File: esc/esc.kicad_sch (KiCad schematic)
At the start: 45 parts, among them IC7 MA702GQ-P, U1 STM32G474RETx, Y1 NX2016SA-24M-EXS00A-CS08891

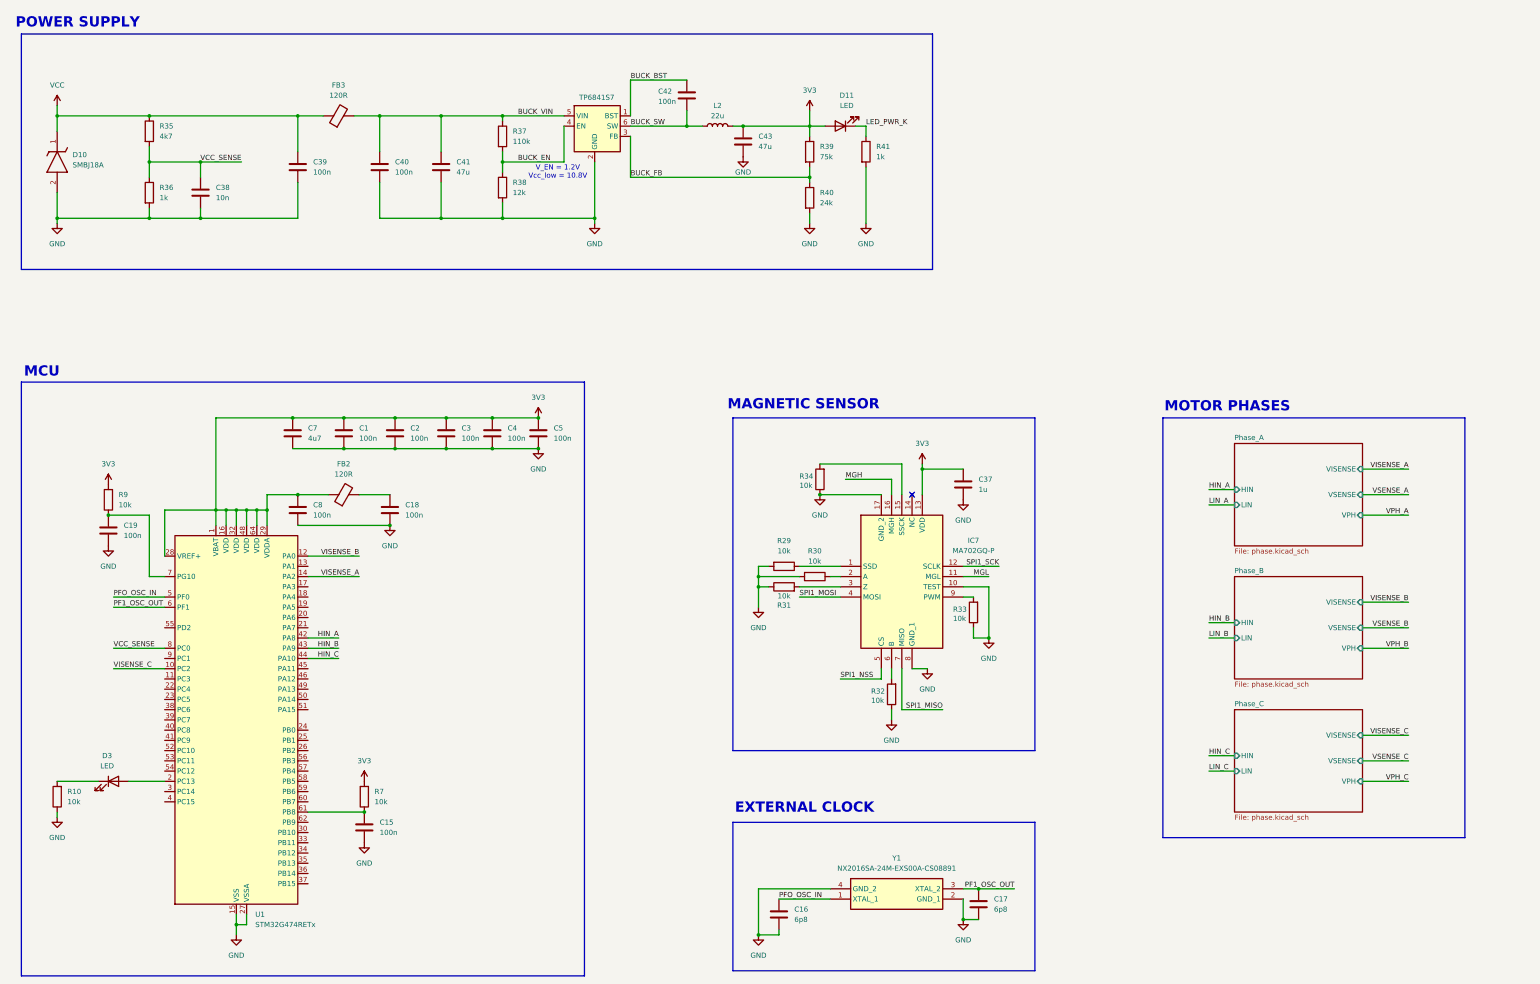
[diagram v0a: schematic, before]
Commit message: full layout
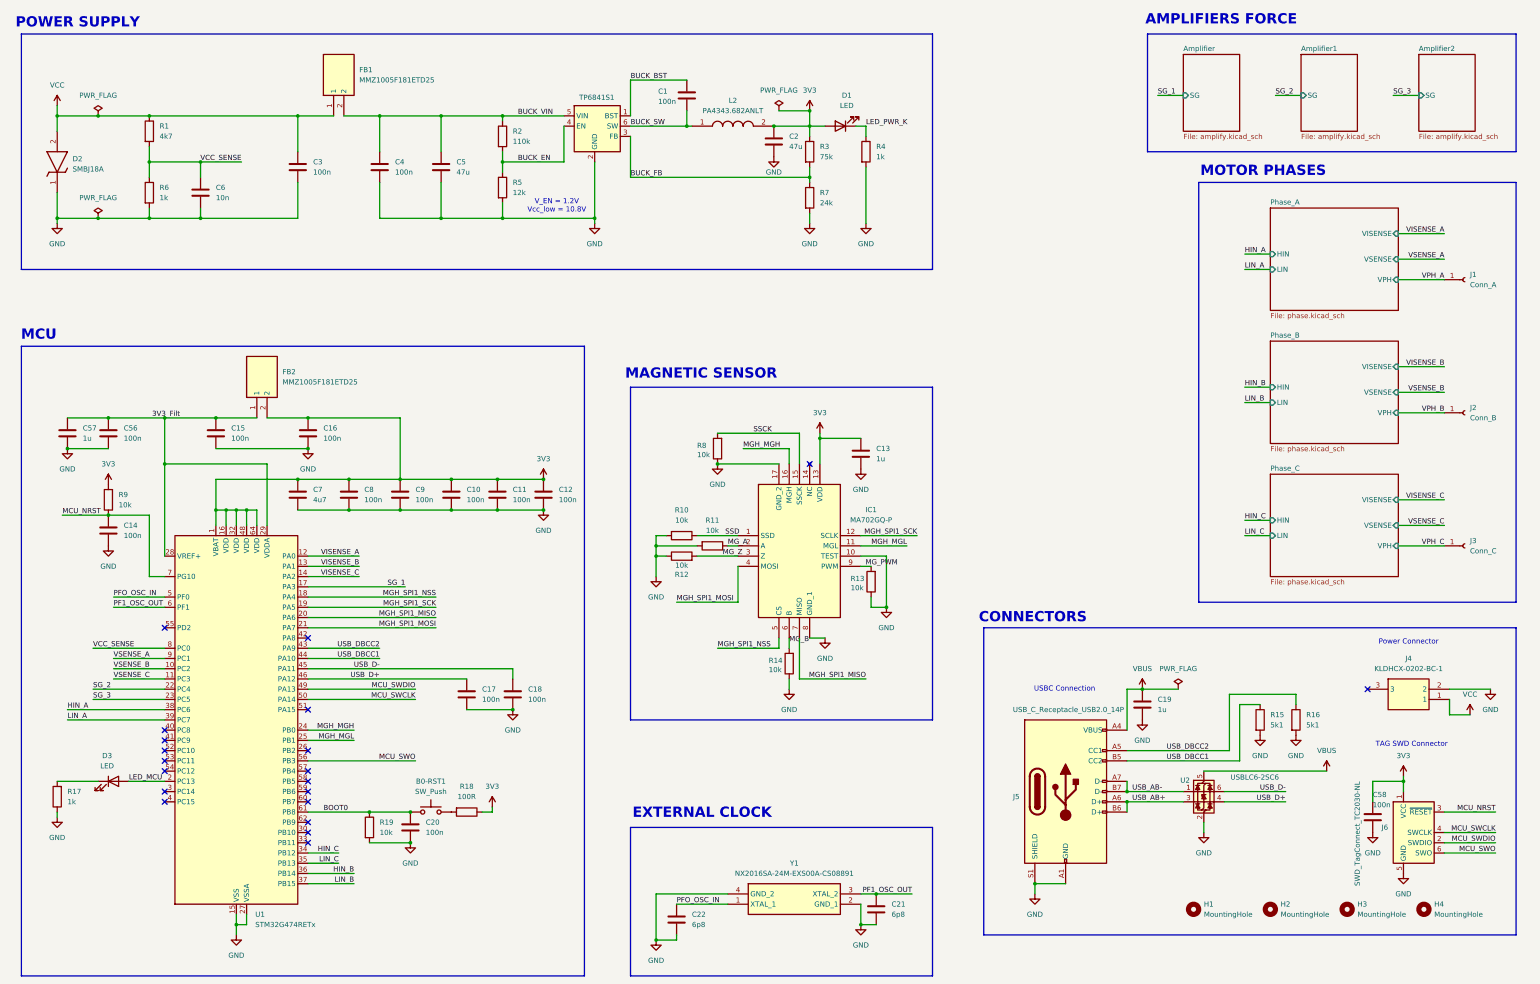
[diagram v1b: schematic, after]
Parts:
- removed D10: SMBJ18A, SamacSys_Parts:SMBJ18A, symbol SamacSys_Parts:SMBJ18A
- removed FB2, FB3: 120R, symbol Device:FerriteBead
- removed IC7: MA702GQ-P, QFN50P300X300X100-17N-D, symbol SamacSys_Parts:MA702GQ-P
- removed L2: 22u, symbol Device:L
- added B0-RST1: SW_Push, Button_Switch_SMD:SW_SPST_B3U-1000P, symbol Switch:SW_Push
- added C17, C18, C56, C58: 100n, Capacitor_SMD:C_0402_1005Metric, symbol Device:C
- added C19, C57: 1u, Capacitor_SMD:C_0603_1608Metric, symbol Device:C
- added D2: SMBJ18A, SamacSys_Parts:DIOM5436X244N, symbol SamacSys_Parts:SMBJ18A
- added FB1, FB2: MMZ1005F181ETD25, SamacSys_Parts:BEADC1005X55N, symbol SamacSys_Parts:MMZ1005F181ETD25
- added H1, H2, H3, H4: MountingHole, MountingHole:MountingHole_3.2mm_M3, symbol Mechanical:MountingHole
- added IC1: MA702GQ-P, SamacSys_Parts:QFN50P300X300X100-17N-D, symbol SamacSys_Parts:MA702GQ-P
- added J1: Conn_A, Connector_Wire:SolderWire-2sqmm_1x01_D2mm_OD3.9mm, symbol Connector:Conn_01x01_Socket
- added J2: Conn_B, Connector_Wire:SolderWire-2sqmm_1x01_D2mm_OD3.9mm, symbol Connector:Conn_01x01_Socket
- added J3: Conn_C, Connector_Wire:SolderWire-2sqmm_1x01_D2mm_OD3.9mm, symbol Connector:Conn_01x01_Socket
- added J4: KLDHCX-0202-BC-1, SamacSys_Parts:KLDHCX0202BC1, symbol SamacSys_Parts:KLDHCX-0202-BC-1
- added J5: USB_C_Receptacle_USB2.0_14P, Connector_USB:USB_C_Receptacle_Amphenol_12401610E4-2A, symbol Connector:USB_C_Receptacle_USB2.0_14P
- added J6: SWD_TagConnect_TC2030-NL, Connector:Tag-Connect_TC2030-IDC-NL_2x03_P1.27mm_Vertical, symbol Connector:Conn_ARM_SWD_TagConnect_TC2030-NL
- added L2: PA4343.682ANLT, SamacSys_Parts:INDPM135126X650N, symbol SamacSys_Parts:PA4343.682ANLT
- added R15, R16: 5k1, Resistor_SMD:R_0603_1608Metric, symbol Device:R
- added R19: 10k, Resistor_SMD:R_0603_1608Metric, symbol Device:R
- added U2: USBLC6-2SC6, Package_TO_SOT_SMD:SOT-23-6, symbol Power_Protection:USBLC6-2SC6
- C1: renamed from C42; footprint (none) -> Capacitor_SMD:C_0402_1005Metric; Link (none) -> https://www.mouser.de/ProductDetail/Murata-Electronics/GRM0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; MF (none) -> Murata Electronics; MP (none) -> GRM02YR60G104ME01L; MPN (none) -> 81-GRM02YR60G104ME1L
- C10: renamed from C3; footprint (none) -> Capacitor_SMD:C_0402_1005Metric; Link (none) -> https://www.mouser.de/ProductDetail/Murata-Electronics/GRM0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; MF (none) -> Murata Electronics; MP (none) -> GRM02YR60G104ME01L; MPN (none) -> 81-GRM02YR60G104ME1L
- C11: renamed from C4; footprint (none) -> Capacitor_SMD:C_0402_1005Metric; Link (none) -> https://www.mouser.de/ProductDetail/Murata-Electronics/GRM0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; MF (none) -> Murata Electronics; MP (none) -> GRM02YR60G104ME01L; MPN (none) -> 81-GRM02YR60G104ME1L
- C12: renamed from C5; footprint (none) -> Capacitor_SMD:C_0402_1005Metric; Link (none) -> https://www.mouser.de/ProductDetail/Murata-Electronics/GRM0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; MF (none) -> Murata Electronics; MP (none) -> GRM02YR60G104ME01L; MPN (none) -> 81-GRM02YR60G104ME1L
- C13: renamed from C37; footprint (none) -> Capacitor_SMD:C_0603_1608Metric; Link (none) -> https://www.mouser.de/ProductDetail/TAIYO-YUDEN/MBJCT168CB7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; MF (none) -> TAIYO YUDEN; MP (none) -> MBJCT168CB7105KRPA01; MPN (none) -> 963-BJCT168CB7105KR
- C14: renamed from C19; footprint (none) -> Capacitor_SMD:C_0402_1005Metric; Link (none) -> https://www.mouser.de/ProductDetail/Murata-Electronics/GRM0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; MF (none) -> Murata Electronics; MP (none) -> GRM02YR60G104ME01L; MPN (none) -> 81-GRM02YR60G104ME1L
- C15: renamed from C8; footprint (none) -> Capacitor_SMD:C_0402_1005Metric; Link (none) -> https://www.mouser.de/ProductDetail/Murata-Electronics/GRM0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; MF (none) -> Murata Electronics; MP (none) -> GRM02YR60G104ME01L; MPN (none) -> 81-GRM02YR60G104ME1L
- C16: renamed from C18; footprint (none) -> Capacitor_SMD:C_0402_1005Metric; Link (none) -> https://www.mouser.de/ProductDetail/Murata-Electronics/GRM0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; MF (none) -> Murata Electronics; MP (none) -> GRM02YR60G104ME01L; MPN (none) -> 81-GRM02YR60G104ME1L
- C2: renamed from C43; footprint (none) -> Capacitor_SMD:C_1206_3216Metric; Link (none) -> https://www.mouser.de/ProductDetail/TDK/C3216X5R1E476M160AC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; MF (none) -> TDK; MP (none) -> C3216X5R1E476M160AC; MPN (none) -> 810-C3216X5R1E476M; Manufacturer_Part_Number (none) -> MLASE31LBB5476MTNA01; Mouser Part Number (none) -> 963-MLASE31LBB5476MT
- C20: renamed from C15; footprint (none) -> Capacitor_SMD:C_0402_1005Metric; Link (none) -> https://www.mouser.de/ProductDetail/Murata-Electronics/GRM0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; MF (none) -> Murata Electronics; MP (none) -> GRM02YR60G104ME01L; MPN (none) -> 81-GRM02YR60G104ME1L
- C21: renamed from C17; footprint (none) -> Capacitor_SMD:C_0402_1005Metric; Link (none) -> https://www.mouser.de/ProductDetail/Murata-Electronics/GJM0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; MF (none) -> Murata Electronics; MP (none) -> GJM0225C1C6R8CB01L; MPN (none) -> 81-GJM0225C1C6R8CB1L
- C22: renamed from C16; footprint (none) -> Capacitor_SMD:C_0402_1005Metric; Link (none) -> https://www.mouser.de/ProductDetail/Murata-Electronics/GJM0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; MF (none) -> Murata Electronics; MP (none) -> GJM0225C1C6R8CB01L; MPN (none) -> 81-GJM0225C1C6R8CB1L
- C3: renamed from C39; footprint (none) -> Capacitor_SMD:C_0402_1005Metric; Link (none) -> https://www.mouser.de/ProductDetail/Murata-Electronics/GRM0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; MF (none) -> Murata Electronics; MP (none) -> GRM02YR60G104ME01L; MPN (none) -> 81-GRM02YR60G104ME1L
- C4: renamed from C40; footprint (none) -> Capacitor_SMD:C_0402_1005Metric; Link (none) -> https://www.mouser.de/ProductDetail/Murata-Electronics/GRM0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; MF (none) -> Murata Electronics; MP (none) -> GRM02YR60G104ME01L; MPN (none) -> 81-GRM02YR60G104ME1L
- C5: renamed from C41; footprint (none) -> Capacitor_SMD:C_1206_3216Metric; Link (none) -> https://www.mouser.de/ProductDetail/TDK/C3216X5R1E476M160AC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; MF (none) -> TDK; MP (none) -> C3216X5R1E476M160AC; MPN (none) -> 810-C3216X5R1E476M; Manufacturer_Part_Number (none) -> MLASE31LBB5476MTNA01; Mouser Part Number (none) -> 963-MLASE31LBB5476MT
- C6: renamed from C38; footprint (none) -> Capacitor_SMD:C_0402_1005Metric; Link (none) -> https://www.mouser.de/ProductDetail/Vishay-Vitramon/VJ0402Y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; MF (none) -> Vishay / Vitramon; MP (none) -> VJ0402Y103KXJAC31X; MPN (none) -> 77-V0402Y103KXJAC31X
- C7: footprint (none) -> Capacitor_SMD:C_0603_1608Metric; Link (none) -> https://www.mouser.de/ProductDetail/TAIYO-YUDEN/MLASE168AB5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; MF (none) -> TAIYO YUDEN; MP (none) -> MLASE168AB5475KTNA01; MPN (none) -> 963-MLASE168AB5475KT
- C8: renamed from C1; footprint (none) -> Capacitor_SMD:C_0402_1005Metric; Link (none) -> https://www.mouser.de/ProductDetail/Murata-Electronics/GRM0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; MF (none) -> Murata Electronics; MP (none) -> GRM02YR60G104ME01L; MPN (none) -> 81-GRM02YR60G104ME1L
- C9: renamed from C2; footprint (none) -> Capacitor_SMD:C_0402_1005Metric; Link (none) -> https://www.mouser.de/ProductDetail/Murata-Electronics/GRM0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; MF (none) -> Murata Electronics; MP (none) -> GRM02YR60G104ME01L; MPN (none) -> 81-GRM02YR60G104ME1L
- D1: renamed from D11; footprint (none) -> LED_SMD:LED_0603_1608Metric; Link (none) -> https://www.mouser.de/ProductDetail/ams-OSRAM/GW-JTLMS3.GM-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; MF (none) -> ams OSRAM; MP (none) -> GW JTLMS3.GM-G3G7-XX58-1-60-R33; MPN (none) -> 720-GWJTLMS3.G3G758
- D3: footprint (none) -> LED_SMD:LED_0603_1608Metric; Link (none) -> https://www.mouser.de/ProductDetail/ams-OSRAM/GW-JTLMS3.GM-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; MF (none) -> ams OSRAM; MP (none) -> GW JTLMS3.GM-G3G7-XX58-1-60-R33; MPN (none) -> 720-GWJTLMS3.G3G758
- R1: renamed from R35; footprint (none) -> Resistor_SMD:R_0603_1608Metric; Link (none) -> https://www.mouser.de/ProductDetail/KOA-Speer/RN73H1ETTP470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; MF (none) -> KOA Speer; MP (none) -> RN73H1ETTP4701D25; MPN (none) -> 660-RN73H1ETP4701D25
- R10: renamed from R29; footprint (none) -> Resistor_SMD:R_0603_1608Metric; Link (none) -> https://www.mouser.de/ProductDetail/Panasonic/ERA-1AEB103C?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; MF (none) -> Panasonic; MP (none) -> ERA-1AEB103C; MPN (none) -> 667-ERA-1AEB103C
- R11: renamed from R30; footprint (none) -> Resistor_SMD:R_0603_1608Metric; Link (none) -> https://www.mouser.de/ProductDetail/Panasonic/ERA-1AEB103C?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; MF (none) -> Panasonic; MP (none) -> ERA-1AEB103C; MPN (none) -> 667-ERA-1AEB103C
- R12: renamed from R31; footprint (none) -> Resistor_SMD:R_0603_1608Metric; Link (none) -> https://www.mouser.de/ProductDetail/Panasonic/ERA-1AEB103C?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; MF (none) -> Panasonic; MP (none) -> ERA-1AEB103C; MPN (none) -> 667-ERA-1AEB103C
- R13: renamed from R33; footprint (none) -> Resistor_SMD:R_0603_1608Metric; Link (none) -> https://www.mouser.de/ProductDetail/Panasonic/ERA-1AEB103C?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; MF (none) -> Panasonic; MP (none) -> ERA-1AEB103C; MPN (none) -> 667-ERA-1AEB103C
- R14: renamed from R32; footprint (none) -> Resistor_SMD:R_0603_1608Metric; Link (none) -> https://www.mouser.de/ProductDetail/Panasonic/ERA-1AEB103C?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; MF (none) -> Panasonic; MP (none) -> ERA-1AEB103C; MPN (none) -> 667-ERA-1AEB103C
- R17: renamed from R10; value 10k -> 1k; footprint (none) -> Resistor_SMD:R_0603_1608Metric; Link (none) -> https://www.mouser.de/ProductDetail/Vishay-Dale/CRCW06031K0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; MF (none) -> Vishay / Dale; MP (none) -> CRCW06031K00FKED; MPN (none) -> 71-CRCW06031K00FKED
- R18: renamed from R7; value 10k -> 100R; footprint (none) -> Resistor_SMD:R_0603_1608Metric; Link (none) -> https://www.mouser.de/ProductDetail/Susumu/RG0603P-101-D-T1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; MF (none) -> Susumu; MP (none) -> RG0603P-101-D-T10; MPN (none) -> 754-RG0603P-101-D
- R2: renamed from R37; footprint (none) -> Resistor_SMD:R_0603_1608Metric; Link (none) -> https://www.mouser.de/ProductDetail/Vishay-Beyschlag/MCT060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; MF (none) -> Vishay / Beyschlag; MP (none) -> MCT06030C1103FP500; MPN (none) -> 594-MCT06030C1103FP5
- R3: renamed from R39; footprint (none) -> Resistor_SMD:R_0603_1608Metric; Link (none) -> https://www.mouser.de/ProductDetail/YAGEO/RT0603FRE1375KL?q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; MF (none) -> YAGEO; MP (none) -> RT0603FRE1375KL; MPN (none) -> 603-RT0603FRE1375KL
- R4: renamed from R41; footprint (none) -> Resistor_SMD:R_0603_1608Metric; Link (none) -> https://www.mouser.de/ProductDetail/Vishay-Dale/CRCW06031K0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; MF (none) -> Vishay / Dale; MP (none) -> CRCW06031K00FKED; MPN (none) -> 71-CRCW06031K00FKED
- R5: renamed from R38; footprint (none) -> Resistor_SMD:R_0603_1608Metric; Link (none) -> https://www.mouser.de/ProductDetail/Vishay-Beyschlag/MCS040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; MF (none) -> Vishay / Beyschlag; MP (none) -> MCS04020D1202BE000; MPN (none) -> 594-MCS04020D1202BE0
- R6: renamed from R36; footprint (none) -> Resistor_SMD:R_0603_1608Metric; Link (none) -> https://www.mouser.de/ProductDetail/Vishay-Dale/CRCW06031K0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; MF (none) -> Vishay / Dale; MP (none) -> CRCW06031K00FKED; MPN (none) -> 71-CRCW06031K00FKED
- R7: renamed from R40; footprint (none) -> Resistor_SMD:R_0603_1608Metric; Link (none) -> https://www.mouser.de/ProductDetail/Panasonic/ERA-3AEB243V?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; MF (none) -> Panasonic; MP (none) -> ERA-3AEB243V; MPN (none) -> 667-ERA-3AEB243V
- R8: renamed from R34; footprint (none) -> Resistor_SMD:R_0603_1608Metric; Link (none) -> https://www.mouser.de/ProductDetail/Panasonic/ERA-1AEB103C?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; MF (none) -> Panasonic; MP (none) -> ERA-1AEB103C; MPN (none) -> 667-ERA-1AEB103C
- R9: footprint (none) -> Resistor_SMD:R_0603_1608Metric; Link (none) -> https://www.mouser.de/ProductDetail/Panasonic/ERA-1AEB103C?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; MF (none) -> Panasonic; MP (none) -> ERA-1AEB103C; MPN (none) -> 667-ERA-1AEB103C
- TP6841S1: renamed from TP6841S7; Link (none) -> https://lcsc.com/product-detail/DC-DC-Converters_TECH-PUBLI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; MF (none) -> TECH PUBLIC; MP (none) -> TP6841S6-A
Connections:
- net 3V3: now also C16.1, R18.1, C58.1, FB2.2, IC1.13 (VDD), J6.1 (VCC), L2.2; no longer C15.1, R18.2, U1.28 (VREF+), U1.29 (VDDA)
- net BUCK_SW: now also L2.1
- net BUCK_VIN: now also FB1.2
- net GND: now also C17.2, C18.2, C19.2, C56.2, C57.2, C58.2, D2.1 (K), IC1.10 (TEST), IC1.17 (GND_2), IC1.8 (GND_1), J4.2, J5.A1 (GND), J5.A12 (GND), J5.B1 (GND), J5.B12 (GND), J5.S1 (SHIELD), J6.5 (GND), R15.2, R16.2, R19.2, U2.2 (GND)
- net HIN_A: now also U1.38 (PC6); no longer U1.42 (PA8)
- net HIN_B: now also U1.36 (PB14); no longer U1.43 (PA9)
- net HIN_C: now also U1.34 (PB12); no longer U1.44 (PA10)
- net LIN_A: now also U1.39 (PC7)
- net LIN_B: now also U1.37 (PB15)
- net LIN_C: now also U1.35 (PB13)
- net VCC: now also D2.2 (A), FB1.1, J4.1
- net VISENSE_A: now also U1.12 (PA0); no longer U1.14 (PA2)
- net VISENSE_B: now also U1.13 (PA1); no longer U1.12 (PA0)
- net VISENSE_C: now also U1.14 (PA2); no longer U1.10 (PC2)
- net VPH_A: now also J1.1 (Pin_1)
- net VPH_B: now also J2.1 (Pin_1)
- net VPH_C: now also J3.1 (Pin_1)
- net VSENSE_A: now also U1.9 (PC1)
- net VSENSE_B: now also U1.10 (PC2)
- net VSENSE_C: now also U1.11 (PC3)
- net LED_MCU: now reaches D3.2 (A), U1.2 (PC13)
- net MG_Z: now reaches R12.2
- net MG_Z: now also IC1.3 (Z)
- net MCU_NRST: now reaches C14.1, R9.1, U1.7 (PG10)
- net MCU_NRST: now also J6.3 (~{RESET})
- net SSD: now reaches R10.1
- net SSD: now also IC1.1 (SSD)
- net SSCK: now reaches R8.2
- net SSCK: now also IC1.15 (SSCK)
- net MG_A: now reaches R11.1
- net MG_A: now also IC1.2 (A)
- net MG_B: now reaches R14.2
- net MG_B: now also IC1.6 (B)
- net MG_PWM: now reaches R13.2
- net MG_PWM: now also IC1.9 (PWM)
- net BOOT0: now reaches C20.1, U1.61 (PB8)
- net BOOT0: now also B0-RST1.1, R19.1; no longer R18.1
- net SG_1: now reaches U1.17 (PA3)
- net MGH_SPI1_NSS: now reaches U1.18 (PA4)
- net MGH_SPI1_NSS: now also IC1.5 (CS)
- net MGH_SPI1_SCK: now reaches U1.19 (PA5)
- net MGH_SPI1_SCK: now also IC1.12 (SCLK)
- net MGH_SPI1_MISO: now reaches U1.20 (PA6)
- net MGH_SPI1_MISO: now also IC1.7 (MISO)
- net MGH_SPI1_MOSI: now reaches U1.21 (PA7)
- net MGH_SPI1_MOSI: now also IC1.4 (MOSI)
- net SG_2: now reaches U1.22 (PC4)
- net SG_3: now reaches U1.23 (PC5)
- net MGH_MGH: now reaches U1.24 (PB0)
- net MGH_MGH: now also IC1.16 (MGH)
- net MGH_MGL: now reaches U1.25 (PB1)
- net MGH_MGL: now also IC1.11 (MGL)
- net USB_D-: now reaches U1.45 (PA11)
- net USB_D-: now also C18.1, U2.6 (I/O1)
- net USB_D+: now reaches U1.46 (PA12)
- net USB_D+: now also C17.1, U2.4 (I/O2)
- net MCU_SWDIO: now reaches U1.49 (PA13)
- net MCU_SWDIO: now also J6.2 (SWDIO)
- net MCU_SWCLK: now reaches U1.50 (PA14)
- net MCU_SWCLK: now also J6.4 (SWCLK)
- net MCU_SWO: now reaches U1.56 (PB3)
- net MCU_SWO: now also J6.6 (SWO)
- new net: B0-RST1.2, R18.2
- new net 3V3_Filt: C15.1, C56.1, C57.1, FB2.1, U1.28 (VREF+), U1.29 (VDDA)
- new net USB_AB+: J5.A6 (D+), J5.B6 (D+), U2.3 (I/O2)
- new net USB_AB-: J5.A7 (D-), J5.B7 (D-), U2.1 (I/O1)
- new net USB_DBCC1: J5.B5 (CC2), R15.1, U1.44 (PA10)
- new net USB_DBCC2: J5.A5 (CC1), R16.1, U1.43 (PA9)
- new net VBUS: C19.1, J5.A4 (VBUS), J5.A9 (VBUS), J5.B4 (VBUS), J5.B9 (VBUS), U2.5 (VBUS)
- no-connect marks 1 -> 20
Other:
- added sheet Amplifier (amplify.kicad_sch)
- added sheet Amplifier1 (amplify.kicad_sch)
- added sheet Amplifier2 (amplify.kicad_sch)
- note added: "AMPLIFIERS FORCE"
- note added: "CONNECTORS"
- note added: "Power Connector"
- note added: "TAG SWD Connector"
- note added: "USBC Connection"
- moved on the sheet: C10, C11, C12, C13, C15, C16, C2, C20, C21, C22, C7, C8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
